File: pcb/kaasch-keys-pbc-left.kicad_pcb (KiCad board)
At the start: 2 copper layers, 73 parts, among them J1 Conn_01x12_Pin, J2 Conn_01x12_Pin, SW1 SW_Push, SW10 SW_Push, SW11 SW_Push, SW12 SW_Push, SW13 SW_Push, SW14 SW_Push, SW15 SW_Push, SW16 SW_Push, SW17 SW_Push, SW18 SW_Push, SW19 SW_Push, SW2 SW_Push, SW20 SW_Push, SW21 SW_Push, SW22 SW_Push, SW23 SW_Push, SW24 SW_Push, SW25 SW_Push, SW26 SW_Push, SW27 SW_Push, SW28 SW_Push, SW29 SW_Push, SW3 SW_Push, SW30 SW_Push, SW31 SW_Push, SW32 SW_Push, SW33 SW_Push, SW34 SW_Push, SW35 SW_Push, SW36 SW_Push_Reset, SW4 SW_Push, SW5 SW_Push, SW6 SW_Push, SW7 SW_Push, SW8 SW_Push, SW9 SW_Push

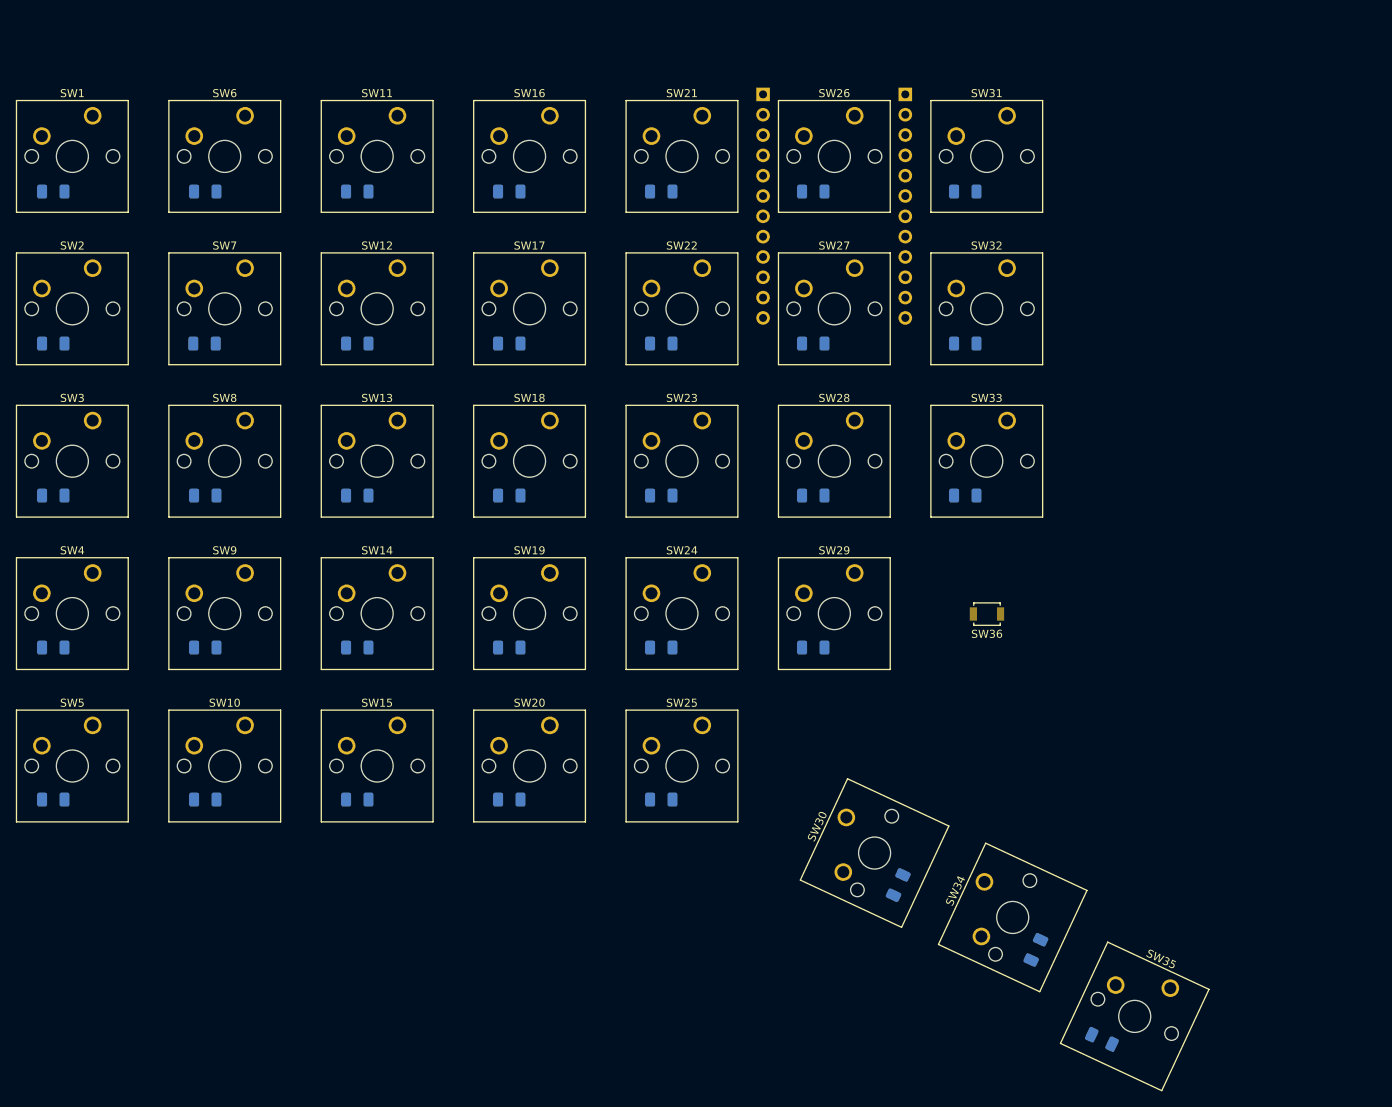
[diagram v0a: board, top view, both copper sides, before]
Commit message: finished new layout
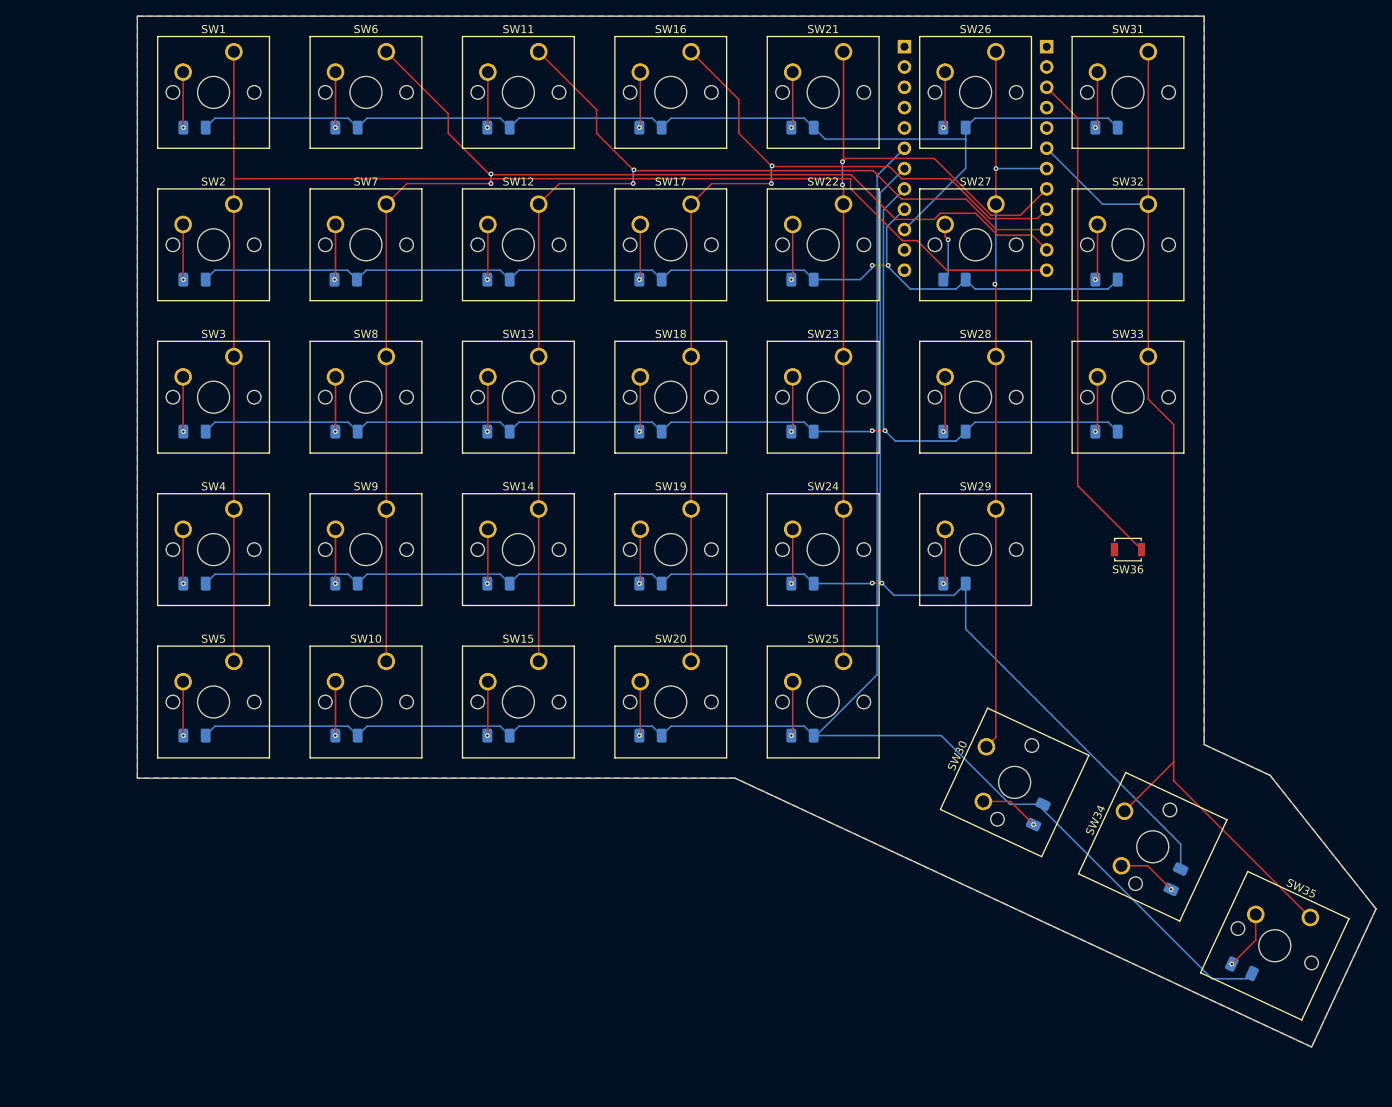
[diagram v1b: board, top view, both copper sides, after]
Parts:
- moved SW30 19.6 mm to (185.0, 125.6)
- moved D30 19.6 mm to (191.5, 134.1)
- moved SW34 19.6 mm to (202.3, 133.7)
- moved SW35 19.6 mm to (225.5, 147.0)
- moved D34 19.6 mm to (208.7, 142.2)
- moved D35 19.6 mm to (216.9, 153.4)
- moved SW36 19.4 mm to (202.7, 101.0)
- moved SW16 19.4 mm to (148.1, 38.8)
- moved SW18 19.4 mm to (148.1, 76.9)
- moved SW19 19.4 mm to (148.1, 95.9)
- moved SW20 19.4 mm to (148.1, 115.0)
- moved SW31 19.4 mm to (205.2, 38.8)
- moved SW33 19.4 mm to (205.2, 76.9)
- moved SW17 19.4 mm to (148.1, 57.8)
- moved SW32 19.4 mm to (205.2, 57.8)
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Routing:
- net row.4.L: track 0.00 -> 226.3 mm
- net row.3.L: track 0.00 -> 200.1 mm, vias 0 -> 2
- net col.0.L: track 0.00 -> 183.3 mm
- net col.1.L: track 0.00 -> 167.4 mm, vias 0 -> 2
- net row.2.L: track 0.00 -> 151.3 mm, vias 0 -> 2
- net col.2.L: track 0.00 -> 146.2 mm, vias 0 -> 2
- net col.6.L: track 0.00 -> 140.9 mm
- net row.0.L: track 0.00 -> 135.4 mm
- net row.1.L: track 0.00 -> 129.8 mm, vias 0 -> 2
- net col.3.L: track 0.00 -> 126.5 mm, vias 0 -> 2
- net col.4.L: track 0.00 -> 106.3 mm, vias 0 -> 2
- net col.5.L: track 0.00 -> 93.8 mm, vias 0 -> 2
- net Net-(J2-Pin_3): track 0.00 -> 62.7 mm
- net Net-(D30-A): track 0.00 -> 7.48 mm, vias 0 -> 1
- net Net-(D34-A): track 0.00 -> 7.44 mm, vias 0 -> 1
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- added copper zone on B.Cu, net GND
- added copper zone on F.Cu, net GND
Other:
- board outline added: 154.8 x 128.9 mm
